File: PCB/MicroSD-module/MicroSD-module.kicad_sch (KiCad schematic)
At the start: 10 parts, among them J1 Connector, K1 HYC77-TF09-200, U1 SE5218, U2 TXB0104PWR

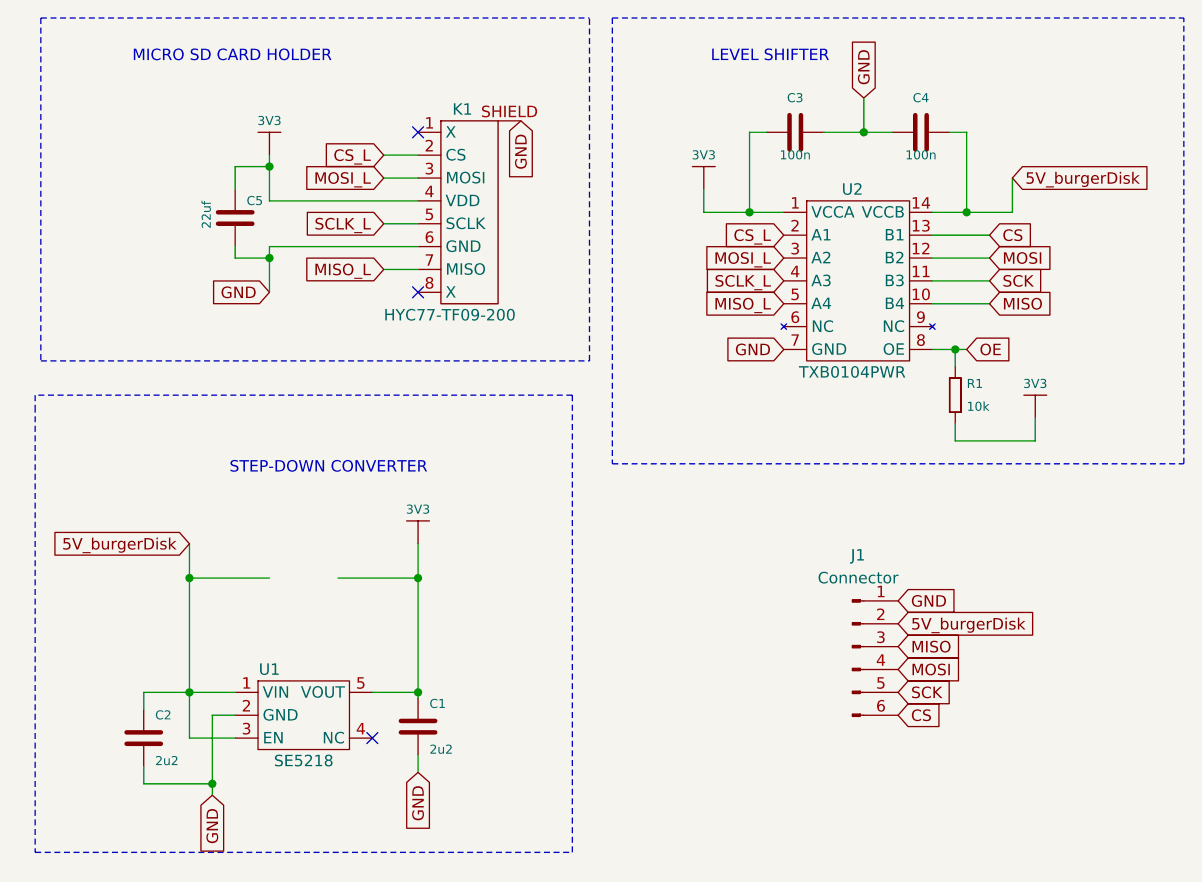
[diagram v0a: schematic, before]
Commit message: Update details
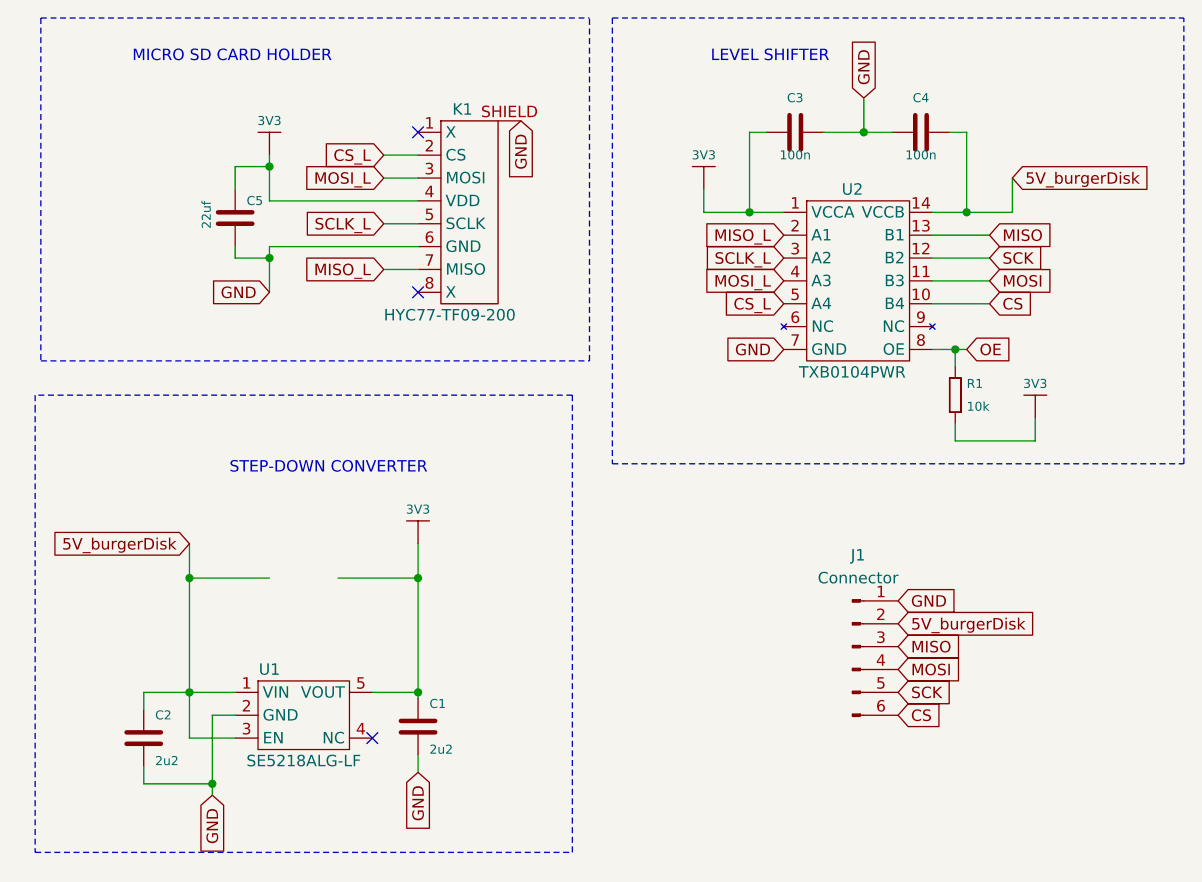
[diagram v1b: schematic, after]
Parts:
- U1: value SE5218 -> SE5218ALG-LF
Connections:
- net CS: now also U2.10 (B4); no longer U2.13 (B1)
- net CS_L: now also U2.5 (A4); no longer U2.2 (A1)
- net MISO: now also U2.13 (B1); no longer U2.10 (B4)
- net MISO_L: now also U2.2 (A1); no longer U2.5 (A4)
- net MOSI: now also U2.11 (B3); no longer U2.12 (B2)
- net MOSI_L: now also U2.4 (A3); no longer U2.3 (A2)
- net SCK: now also U2.12 (B2); no longer U2.11 (B3)
- net SCLK_L: now also U2.3 (A2); no longer U2.4 (A3)
